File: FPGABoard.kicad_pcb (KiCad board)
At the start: 2 copper layers, 100 x 80 mm, 76 parts, among them P1 JTAG_FPGA, P3 USB_B, P4 CONN_02X07, P5 JTAG, P6 CONN_02X07, P7 CONN_02X07, P8 CONN_02X07, Q1 Q_NMOS_DSG, SW1 SW_PUSH, SW2 SW_PUSH, U1 XC3S50A/VQ100, U2 LM317_SOT223, U3 LM317_SOT223, U4 LM317_SOT223, U5 ATMEGA32U4RC-A, U6 M25P20, Y1 12MHz

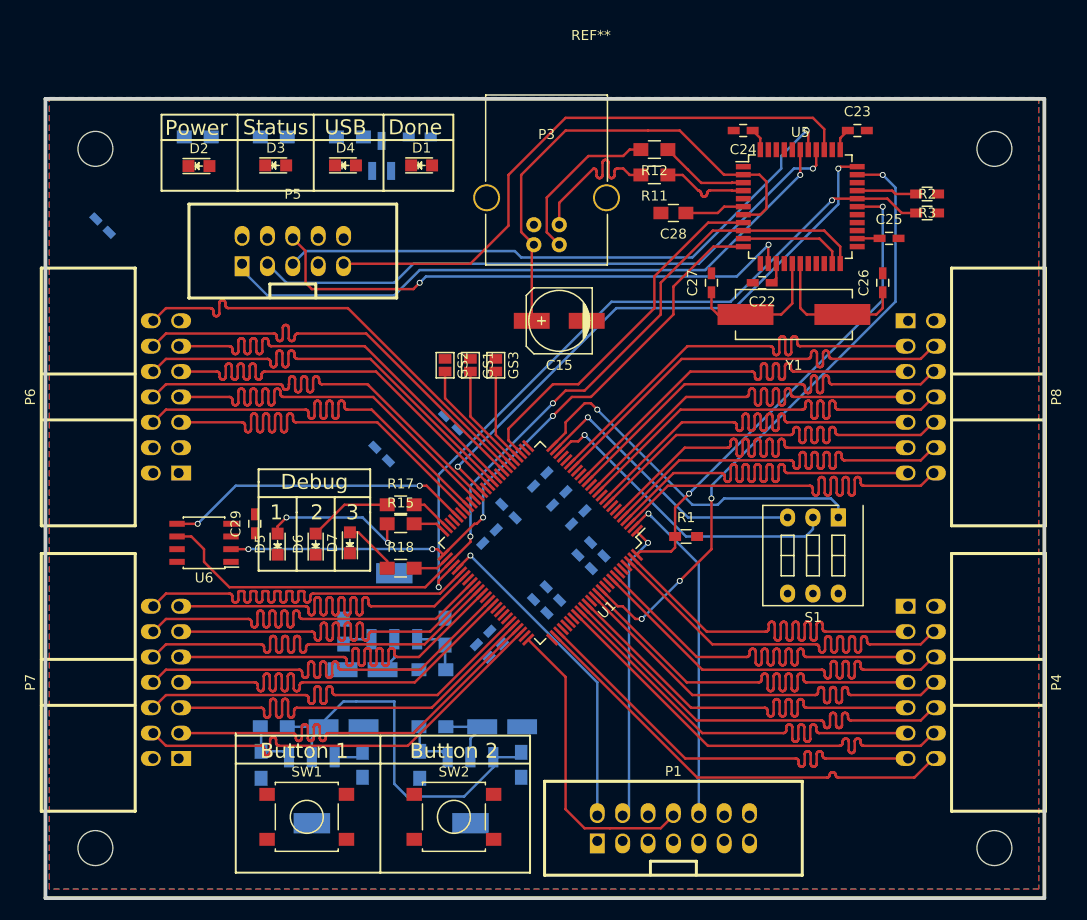
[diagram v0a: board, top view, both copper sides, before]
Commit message: Layouting
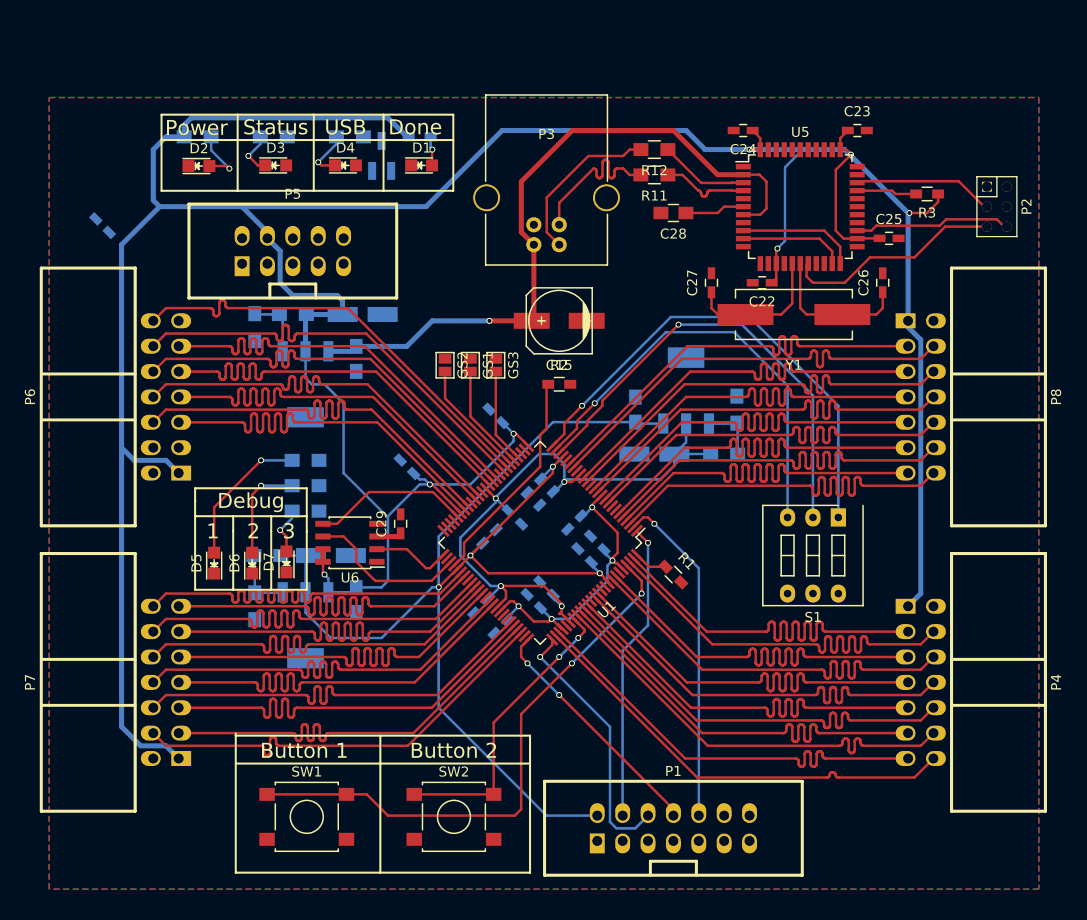
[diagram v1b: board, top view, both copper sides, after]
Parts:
- removed REF**: EuroBoard_halb_Type-I_100mmX80mm_holes, EuroBoard_Outline:EuroBoard_halb_Type-I_100mmX80mm_holes
- added P2: CONN_02X03, w_pin_strip:pin_strip_3x2, F.Cu at (183.5, 71.8)
- R15, R17, R18: moved to B.Cu
- moved R8 43.8 mm to (109.2, 83.8)
- moved C17 41.3 mm to (120.0, 82.5)
- moved R4 41.3 mm to (113.0, 82.5)
- moved U2 40.6 mm to (114.3, 89.5)
- moved C16 40.6 mm to (119.4, 87.0)
- moved R2 40.6 mm to (139.7, 89.5)
- moved C20 36.7 mm to (147.3, 92.1)
- moved R10 36.7 mm to (157.5, 92.1)
- moved R6 36.3 mm to (156.2, 96.5)
- moved U4 36.3 mm to (152.4, 90.2)
- moved C21 36.3 mm to (149.2, 96.5)
- moved C19 24.2 mm to (116.8, 106.7)
- moved R5 23.8 mm to (110.5, 106.7)
- moved U3 23.3 mm to (114.3, 113.7)
- moved C18 23.3 mm to (119.4, 111.1)
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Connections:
- U1 pad 82: (no net) -> /Connections/BTN2
- U1 pad 97: (no net) -> /Connections/BTN1
- U5 pad 18: (no net) -> /Connections/C_IO2
- U5 pad 19: (no net) -> /Connections/C_IO3
- U5 pad 25: (no net) -> /Connections/C_IO4
- U5 pad 31: (no net) -> /Connections/C_IO1
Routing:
- net VCC: track 48.4 -> 389.7 mm, vias 0 -> 11
- net VCC_AUX: track 43.3 -> 128.4 mm, vias 1 -> 4
- net Net-(P5-Pad1): track 65.1 -> 0.64 mm, vias 1 -> 0
- net /Microcontroller/SCK: track 91.5 -> 28.2 mm, vias 2 -> 0
- net /Spartan3A/Clock_In: track 63.3 -> 0.00 mm, vias 4 -> 0
- net Net-(P5-Pad3): track 62.2 -> 0.00 mm, vias 1 -> 0
- net Net-(P5-Pad5): track 60.2 -> 0.00 mm, vias 1 -> 0
- net /Microcontroller/MISO: track 67.8 -> 8.01 mm, vias 4 -> 0
- net Net-(P5-Pad9): track 59.7 -> 0.00 mm
- net VCC_INT: track 7.17 -> 65.7 mm, vias 0 -> 4
- net /Microcontroller/CS_FPGA: track 58.2 -> 0.07 mm, vias 2 -> 0
- net /Connections/BTN1: track 0.00 -> 56.6 mm, vias 0 -> 2
- net /Microcontroller/RESET: track 55.3 -> 0.00 mm, vias 2 -> 0
- net /Microcontroller/DONE: track 73.9 -> 22.1 mm, vias 2 -> 0
- net /Microcontroller/PROG_B: track 49.4 -> 3.36 mm, vias 2 -> 0
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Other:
- board outline removed
- net class Supply added: clearance 0.1, trace_width 0.5, via_dia 0.6, via_drill 0.4

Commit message: Layout
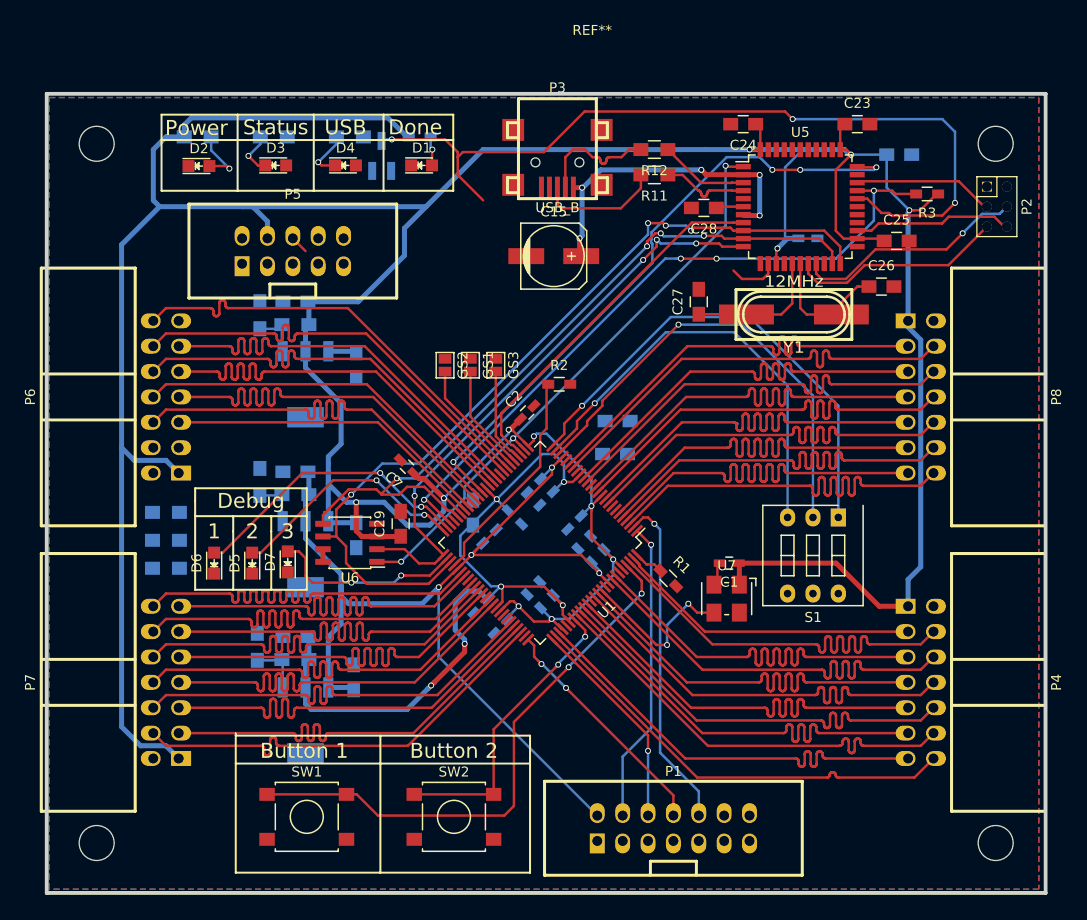
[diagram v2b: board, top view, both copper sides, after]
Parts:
- added C30: 1µF, Capacitors_SMD:C_0805_HandSoldering, B.Cu at (131.1, 102.4)
- added C31: 1µF, Capacitors_SMD:C_0805_HandSoldering, B.Cu at (173.7, 66.5)
- added C32: 1µF, Capacitors_SMD:C_0805_HandSoldering, B.Cu at (145.5, 93.2)
- added C33: 1µF, Capacitors_SMD:C_0805_HandSoldering, B.Cu at (145.3, 96.5)
- added REF**: EuroBoard_halb_Type-I_100mmX80mm_holes, EuroBoard_Outline:EuroBoard_halb_Type-I_100mmX80mm_holes, F.Cu at (88.4, 140.5)
- added U7: XO53, Oscillator__Crystal_SMD:Oscillator_XO53, F.Cu at (156.5, 111.0)
- C1, C2, C7: moved to F.Cu
- C17, C19, C21: footprint Capacitors_Tantalum_SMD:TantalC_SizeA_EIA-3216_HandSoldering -> Capacitors_SMD:C_0805_HandSoldering
- C22: moved to B.Cu
- C23, C24, C25, C26, C27, C29: footprint Capacitors_SMD:C_0603_HandSoldering -> Capacitors_SMD:C_0805_HandSoldering
- P3: footprint Connect:USB_B -> w_conn_pc:conn_usb_B_mini_smd
- Y1: footprint Crystals:Crystal_HC49-SD_SMD -> w_crystal:hc-49_smd
- moved C1 71.3 mm to (156.7, 107.4), turned to 180 degrees
- moved R10 53.6 mm to (109.5, 115.8)
- moved U4 50.4 mm to (114.3, 123.2), turned to 0 degrees
- moved R6 47.6 mm to (113.3, 117.1), turned to 180 degrees
- moved C21 40.3 mm to (113.3, 114.8)
- moved C20 38.9 mm to (119.1, 118.9)
- moved R18 15.1 mm to (100.3, 108.0)
- moved R17 15.0 mm to (100.3, 105.2)
- moved R15 14.9 mm to (100.3, 102.4)
- moved R9 12.5 mm to (109.7, 99.3), turned to 90 degrees
- moved P3 9.90 mm to (139.5, 66.0), turned to 180 degrees
- moved C19 9.11 mm to (113.3, 98.3), turned to 180 degrees
- moved U3 7.11 mm to (114.3, 106.6)
- moved C17 6.85 mm to (113.3, 81.3), turned to 180 degrees
- moved R5 6.71 mm to (113.3, 100.6)
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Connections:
- D5 pad 1: GND -> Net-(D5-Pad1)
- D5 pad 2: Net-(D5-Pad2) -> /Connections/LED2
- D6 pad 1: GND -> Net-(D6-Pad1)
- D6 pad 2: Net-(D6-Pad2) -> /Connections/LED1
- D7 pad 1: GND -> Net-(D7-Pad1)
- D7 pad 2: Net-(D7-Pad2) -> /Connections/LED3
- P2 pad 1: (no net) -> VCC
- P2 pad 2: (no net) -> GND
- R1 pad 1: /Microcontroller/PROG_B -> Net-(R1-Pad1)
- R15 pad 1: Net-(D5-Pad2) -> GND
- R15 pad 2: /Connections/LED2 -> Net-(D6-Pad1)
- R17 pad 1: Net-(D6-Pad2) -> GND
- R17 pad 2: /Connections/LED1 -> Net-(D5-Pad1)
- R18 pad 1: Net-(D7-Pad2) -> GND
- R18 pad 2: /Connections/LED3 -> Net-(D7-Pad1)
- U1 pad 100: /Microcontroller/PROG_B -> Net-(R1-Pad1)
- U1 pad 90: /Spartan3A/Clock_In -> Net-(U1-Pad90)
- U5 pad 28: /Microcontroller/PROG_B -> (no net)
- U5 pad 32: /Spartan3A/Clock_In -> (no net)
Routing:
- net /Microcontroller/DONE: track 22.1 -> 107.0 mm, vias 0 -> 3
- net /Microcontroller/CS_FPGA: track 0.07 -> 63.8 mm, vias 0 -> 4
- net /Microcontroller/INIT_B: track 6.04 -> 69.3 mm, vias 0 -> 4
- net /Microcontroller/CS_FLASH: track 0.47 -> 59.4 mm, vias 0 -> 3
- net /Microcontroller/SCK: track 28.2 -> 85.7 mm, vias 0 -> 4
- net /Microcontroller/MISO: track 8.01 -> 59.3 mm, vias 0 -> 4
- net /Microcontroller/MOSI: track 26.5 -> 75.5 mm, vias 0 -> 4
- net /Microcontroller/CS_C: track 0.00 -> 37.1 mm
- net VCC: track 389.7 -> 425.3 mm, vias 11 -> 12
- net /Microcontroller/V_USB: track 70.5 -> 35.2 mm, vias 1 -> 5
- net /Connections/LED1: track 0.00 -> 28.9 mm, vias 0 -> 2
- net /Connections/LED2: track 0.00 -> 24.2 mm, vias 0 -> 2
- net /Connections/C_IO3: track 0.00 -> 23.3 mm, vias 0 -> 1
- net VCC_AUX: track 128.4 -> 105.5 mm
- net /Connections/LED3: track 0.00 -> 20.0 mm, vias 0 -> 2
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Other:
- board outline added: 100 x 80 mm
